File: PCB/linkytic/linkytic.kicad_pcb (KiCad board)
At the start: 2 copper layers, 29.5 x 57 mm, 15 parts, among them J1 L2, J2 L1, J3 A, SW1 SW_Push_Open, U1 M5333B, U2 E18-MS1-PCB, U3 CC_debugger

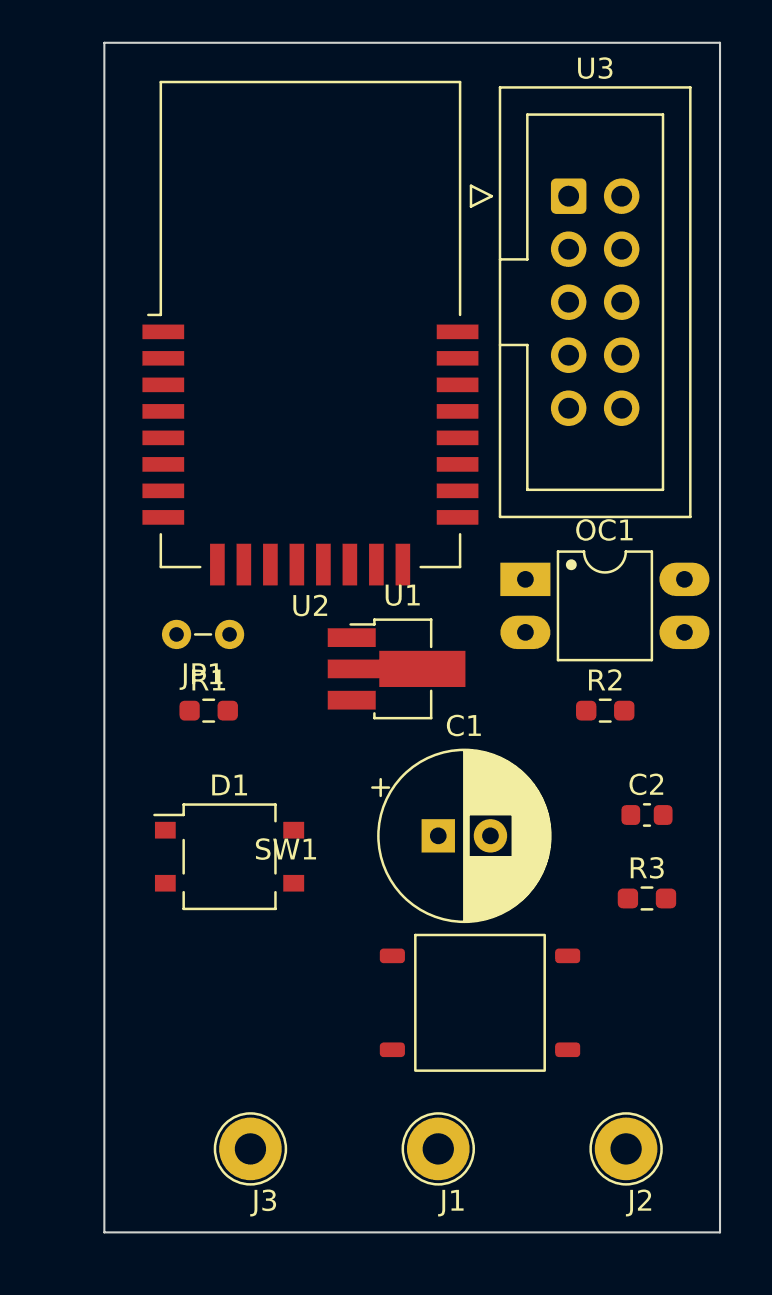
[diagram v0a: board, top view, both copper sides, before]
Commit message: first version, that will notwork :/
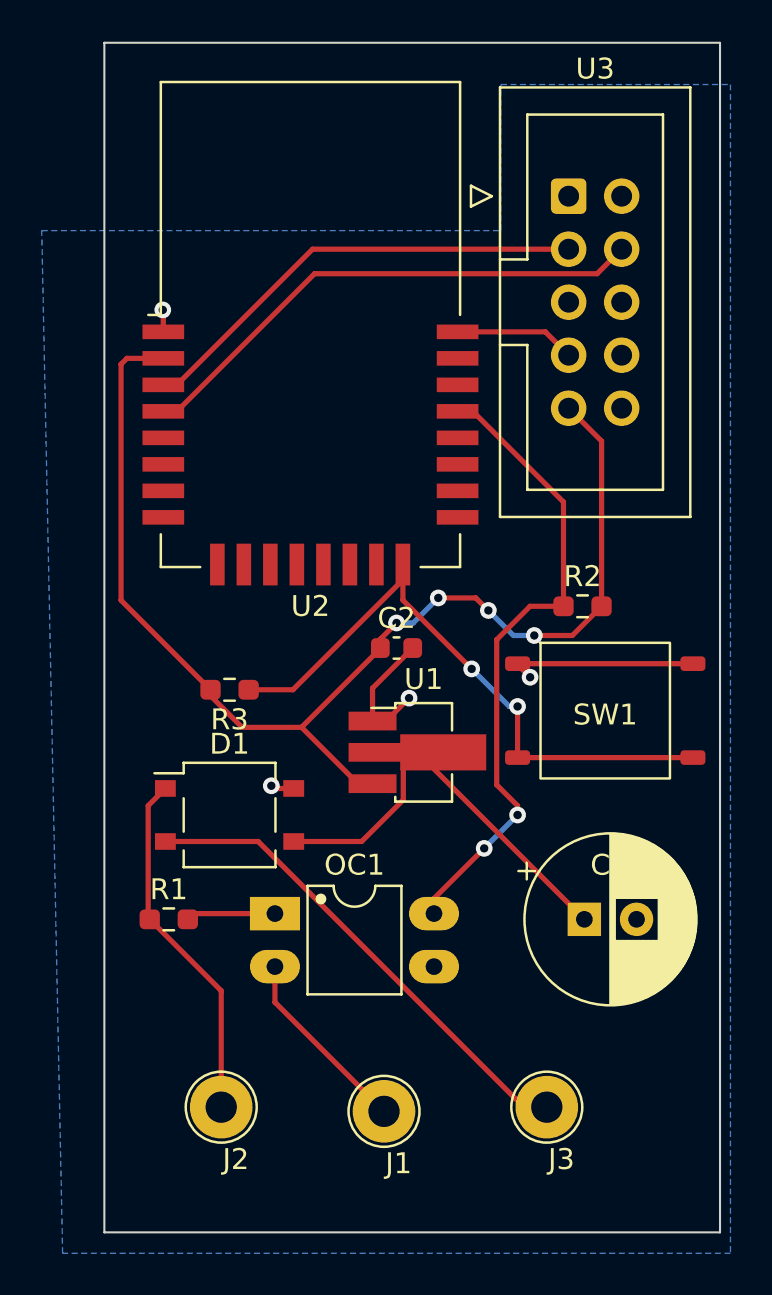
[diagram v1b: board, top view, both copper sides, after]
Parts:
- removed JP1: Jumper_2_Open, Jumper_AKL:Jumper_P2.54mm_D0.7mm
- SW1: value SW_Push_Open -> benoit
- moved R3 22.4 mm to (49.0, 69.0), turned to 180 degrees
- moved OC1 20.0 mm to (51.2, 79.7)
- moved J2 19.5 mm to (48.6, 89.0)
- moved SW1 15.2 mm to (62.8, 67.8)
- moved C2 14.4 mm to (57.0, 67.0)
- moved J3 14.3 mm to (64.2, 89.0)
- moved R1 10.2 mm to (46.1, 80.0)
- moved C1 8.06 mm to (66.0, 80.0)
- moved R2 5.12 mm to (65.9, 65.0)
- moved U1 4.12 mm to (58.0, 72.0)
- moved J1 3.16 mm to (56.4, 89.2)
- moved D1 2.00 mm to (49.0, 75.0)
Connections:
- R3 pad 2: Net-(JP1-Pad2) -> 3v3
- U2 pad 2: Net-(JP1-Pad2) -> 3v3
- U3 pad 9: Net-(JP1-Pad2) -> 3v3
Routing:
- net 3v3: track 0.00 -> 58.0 mm, vias 0 -> 4
- net Net-(OC1-Pad4): track 0.00 -> 30.9 mm, vias 0 -> 2
- net Net-(R3-Pad1): track 0.00 -> 30.5 mm, vias 0 -> 2
- net Net-(U2-Pad4): track 0.00 -> 25.2 mm
- net Net-(D1-Pad2): track 0.00 -> 23.5 mm
- net Net-(U2-Pad3): track 0.00 -> 22.1 mm
- net Net-(C1-Pad1): track 0.00 -> 21.0 mm
- net GND: track 0.00 -> 18.0 mm, vias 0 -> 4
- net Net-(D1-Pad1): track 0.00 -> 17.1 mm
- net Net-(J1-Pad1): track 0.00 -> 9.10 mm
- net Net-(U2-Pad24): track 0.00 -> 5.79 mm
- net Net-(OC1-Pad1): track 0.00 -> 4.29 mm
- added copper zone on B.Cu, net GND
